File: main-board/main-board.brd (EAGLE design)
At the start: 91.4 x 59.4 mm, 142 parts, among them IC1 MEGA8-AI, IC2 LMV324M, IC3 4051D, IC4 4051D, IC6 74HC595D, IC8 74AC14D

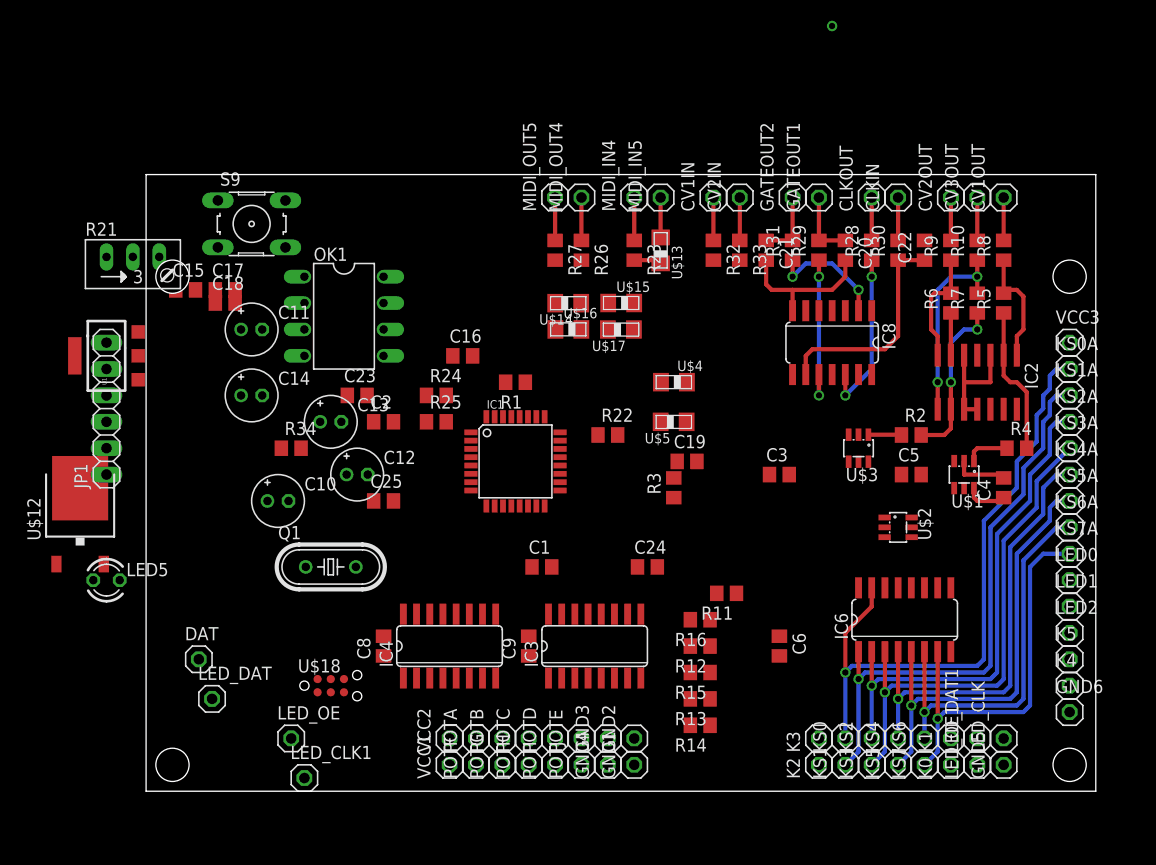
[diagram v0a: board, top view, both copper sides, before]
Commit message: mode mods
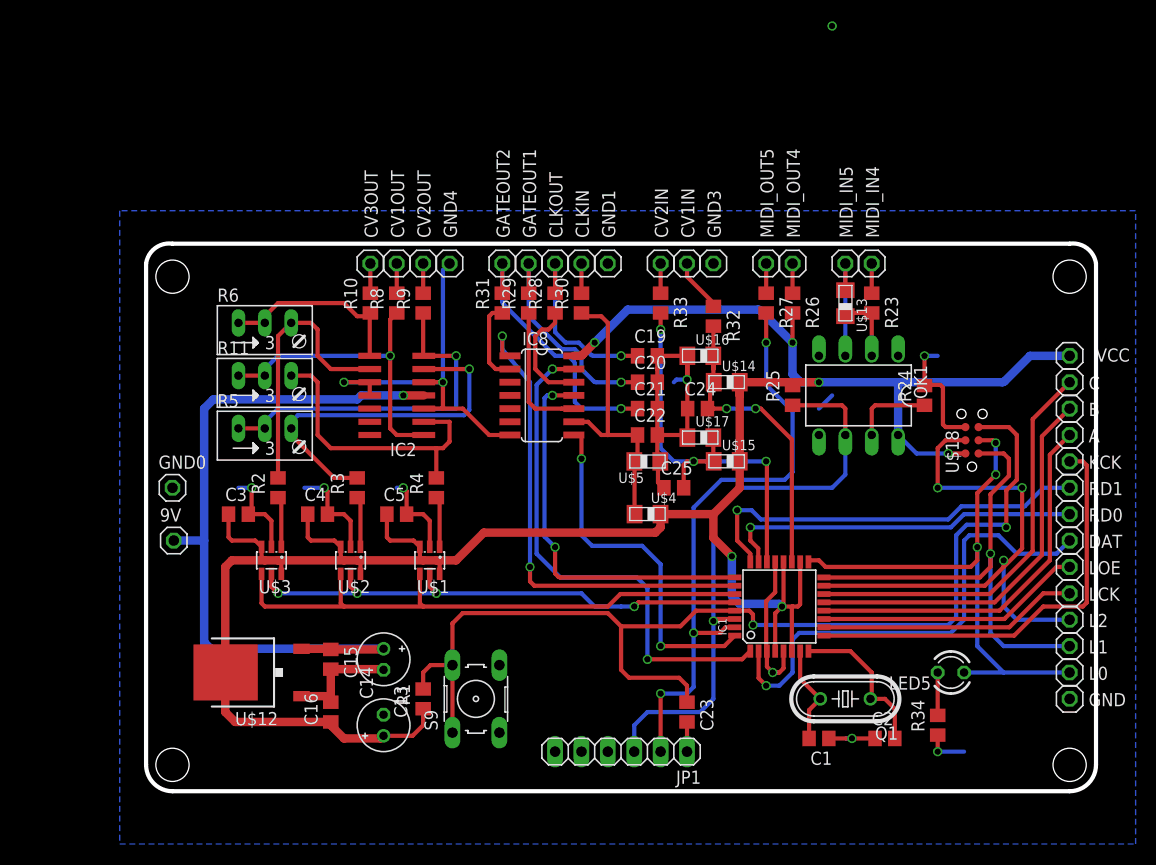
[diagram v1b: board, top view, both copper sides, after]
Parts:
- removed C10, C11, C12: (no value), rcl:E2-5
- removed C17, C18, C6, C8, C9: (no value), rcl:C0805
- removed GND2, GND5, GND6, K0, K1, K2, K3, K4, K5, KS0, KS0A, KS1, KS1A, KS2, KS2A, KS3, KS3A, KS4, KS4A, KS5, KS5A, KS6, KS6A, KS7, KS7A, LED0, LED1, LED2, LED_CLK, LED_CLK1, LED_DAT, LED_DAT1, LED_OE, LED_OE1, POTA, POTB, POTC, POTD, POTE, POTF, POTG, POTH, POTI, POTJ, VCC1, VCC2, VCC3: (no value), pinhead:1X01
- removed IC3, IC4: 4051D, 40xx:SO16
- removed IC6: 74HC595D, 74xx-eu:SO16
- removed R12, R13, R14, R15, R16, R22, R7: (no value), rcl:R0805
- removed R21: (no value), pot:RJ9W
- removed U1: (no value), microbuilder:SOT223-R
- added 9V, A, B, C, GND, GND0, KCK, L0, L1, L2, LCK, LOE, RD0, RD1, VCC: (no value), pinhead:1X01
- IC2: value LMV324M -> LM324D
- R11, R5, R6: device rcl:R0805 -> pot:RJ9W
- moved DAT 84.6 mm to (99.1, 26.7)
- moved LED5 81.8 mm to (87.6, 14.0), turned to 180 degrees
- moved R5 72.2 mm to (21.6, 36.8), turned to 0 degrees
- moved R34 67.7 mm to (86.4, 8.89), turned to 90 degrees
- moved U$18 67.6 mm to (89.7, 33.8), turned to 90 degrees
- moved C4 66.1 mm to (26.7, 29.2), turned to 0 degrees
- moved R6 66.1 mm to (21.6, 47.0), turned to 0 degrees
- moved R2 61.2 mm to (22.9, 31.8), turned to 90 degrees
- moved JP1 59.5 mm to (55.9, 6.35), turned to 180 degrees
- moved CV3OUT 58.8 mm to (31.8, 53.3)
- moved CV1OUT 58.8 mm to (34.3, 53.3)
- moved R10 58.6 mm to (31.8, 49.5)
- moved R8 58.6 mm to (34.3, 49.5)
- moved U$3 57.5 mm to (22.2, 24.8)
- moved C2 57.1 mm to (81.3, 7.62)
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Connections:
- removed net N$16: IC3.5, K0.1, R16.2
- removed net N$18: IC3.1, POTE.1
- removed net N$19: IC3.12, POTD.1
- removed net N$20: IC3.15, POTC.1
- removed net N$21: IC3.14, POTB.1
- removed net N$22: IC3.13, POTA.1
- removed net N$23: IC4.4, K5.1
- removed net N$24: IC4.2, K4.1, R11.2
- removed net N$26: IC6.2, KS2.1, KS2A.1
- removed net N$27: IC6.3, KS3.1, KS3A.1
- removed net N$28: IC6.4, KS4.1, KS4A.1
- removed net N$29: IC6.5, KS5.1, KS5A.1
- removed net N$30: IC6.6, KS6.1, KS6A.1
- removed net N$31: IC6.7, KS7.1, KS7A.1
- removed net N$32: IC4.5, K3.1, R12.2
- removed net N$33: IC4.1, POTJ.1, R13.2
- removed net N$34: IC4.12, POTI.1
- removed net N$35: IC4.15, POTH.1
- removed net N$36: IC4.14, POTG.1
- removed net N$37: IC4.13, POTF.1
- removed net N$38: LED_DAT.1, LED_DAT1.1
- removed net N$5: IC6.1, KS1.1, KS1A.1
- removed net N$50: IC6.15, KS0.1, KS0A.1
- removed net N$55: C11.+, R21.E, R21.S, R22.2, U1.1
- removed net N$8: IC3.4, K2.1, R14.2
- removed net N$9: IC3.2, K1.1, R15.2
- removed net READ0: IC1.23, IC3.3
- removed net READ1: IC1.24, IC4.3
- removed net VREF: C12.+, C17.1, IC2.4, R22.1, U1.2
- new net RD0: IC1.23, RD0.1
- new net RD1: IC1.24, RD1.1
- net 1: now also L2.1; no longer LED2.1
- net 2: now also L1.1; no longer LED1.1
- net 3: now also L0.1; no longer LED0.1
- net 9V: now also 9V.1, IC2.4; no longer C10.+, C18.1, U1.3
- net DAT: no longer IC6.14
- net GND: now also GND.1, GND0.1; no longer C10.-, C11.-, C12.-, C17.2, C18.2, C6.2, C8.2, C9.2, GND2.1, GND5.1, GND6.1, IC3.6, IC3.7, IC3.8, IC4.6, IC4.7, IC4.8, IC6.13, IC6.8, R11.1, R12.1, R13.1, R14.1, R15.1, R16.1, R21.A
- net KS_CLK: now also KCK.1; no longer IC6.11, IC6.12
- net LED_CLK: now also LCK.1; no longer LED_CLK.1, LED_CLK1.1
- net LED_OE: now also LOE.1; no longer LED_OE.1, LED_OE1.1
- net N$10: now also R5.A; no longer R6.1
- net N$11: now also R6.E, R6.S; no longer R7.2
- net N$12: now also R5.E, R5.S; no longer R6.2
- net N$17: now also R11.E, R11.S; no longer R5.2
- net N$3: no longer U$17.A
- net N$4: now also U$17.A
- net N$6: now also R11.A; no longer R5.1
- net N$7: now also R6.A; no longer R7.1
- net SELA: now also A.1; no longer IC3.11, IC4.11
- net SELB: now also B.1; no longer IC3.10, IC4.10
- net SELC: now also C.1; no longer IC3.9, IC4.9
- net VCC: now also VCC.1; no longer C6.1, C8.1, C9.1, IC3.16, IC4.16, IC6.10, IC6.16, VCC1.1, VCC2.1, VCC3.1
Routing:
- net VCC: track 4.23 -> 239.8 mm, vias 0 -> 6
- net GND: track 31.1 -> 145.2 mm, vias 0 -> 10
- net RESET: track 0.00 -> 106.0 mm, vias 0 -> 2
- net 9V: track 0.00 -> 72.6 mm, vias 0 -> 1
- net N$50: track 61.5 -> 0.00 mm, vias 1 -> 0
- net MIDI_OUT: track 0.00 -> 57.8 mm, vias 0 -> 3
- net MIDI_IN: track 0.00 -> 57.0 mm, vias 0 -> 1
- net SDA: track 0.00 -> 55.6 mm
- net N$5: track 54.6 -> 0.00 mm, vias 1 -> 0
- net 3: track 0.00 -> 53.9 mm, vias 0 -> 3
- net 1: track 0.00 -> 53.3 mm, vias 0 -> 3
- net SCL: track 0.00 -> 51.1 mm, vias 0 -> 4
- net CLKOUT: track 0.00 -> 49.6 mm, vias 0 -> 2
- net N$26: track 48.7 -> 0.00 mm, vias 1 -> 0
- net N$27: track 48.2 -> 0.00 mm, vias 1 -> 0
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- added copper zone on layer 16, net GND
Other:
- board size 91.4 x 59.4 mm -> 91.4 x 52.7 mm
